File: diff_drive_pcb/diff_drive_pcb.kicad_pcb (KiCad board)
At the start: 2 copper layers, 13 parts, among them J1 Conn_01x02_Pin, J10 Conn_01x02_Pin, J2 Conn_01x04_Socket, J3 Conn_01x02_Pin, J4 Conn_01x04_Socket, J5 Conn_01x02_Pin, J6 Conn_01x04_Socket, J7 Conn_01x02_Pin, J8 Conn_01x04_Socket, J9 Conn_01x02_Pin, U1 TB6612FNG, U2 TB6612FNG, U3 Teensy4.1

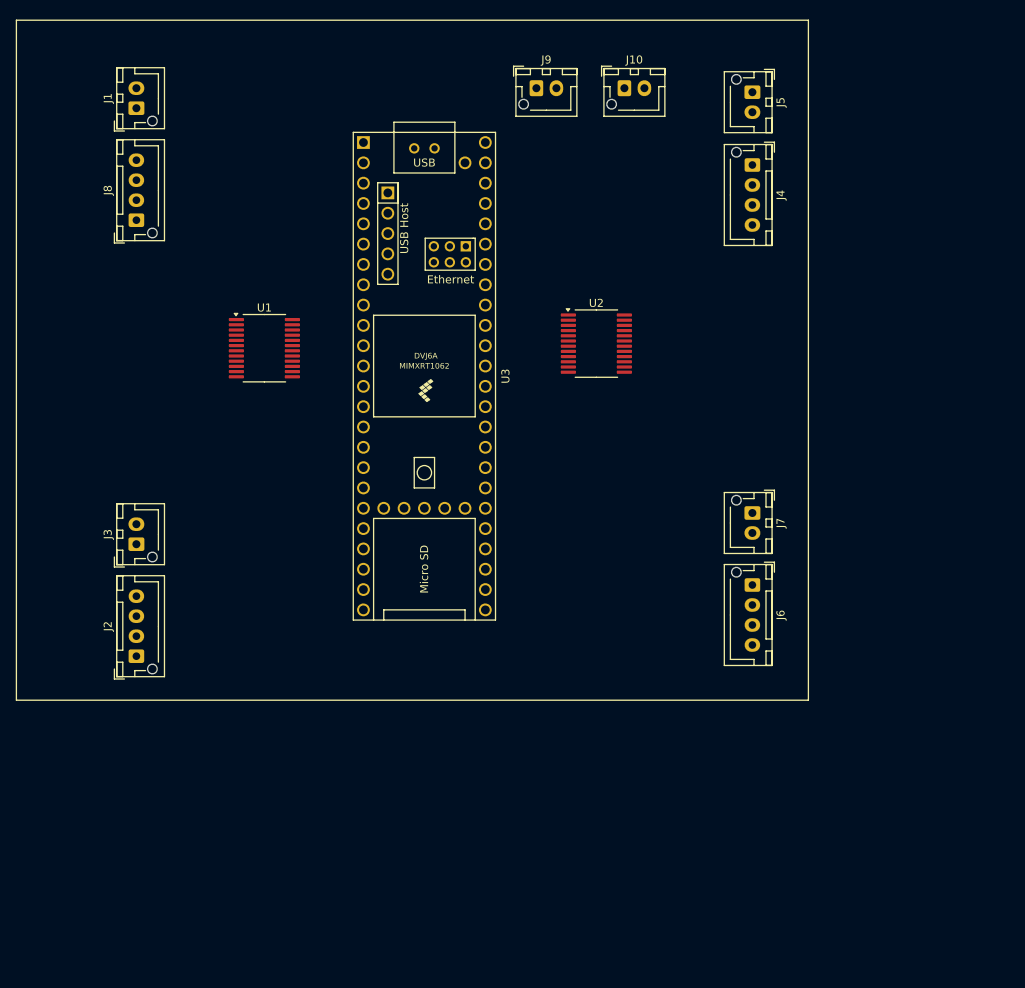
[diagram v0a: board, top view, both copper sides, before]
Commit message: PCB v1.0 developed
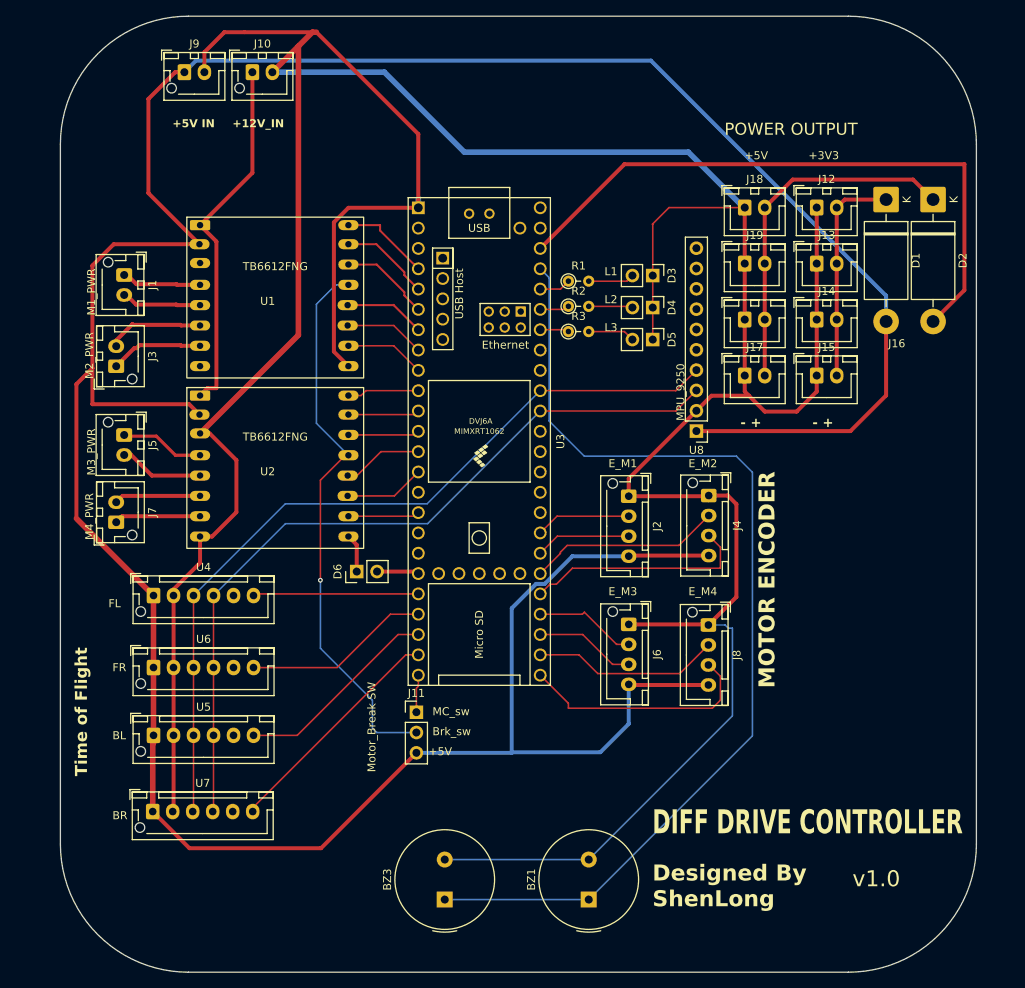
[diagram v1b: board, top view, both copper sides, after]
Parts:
- added BZ1: Buzzer, Buzzer_Beeper:Buzzer_TDK_PS1240P02BT_D12.2mm_H6.5mm, F.Cu at (167.5, 143.9)
- added BZ3: Buzzer, Buzzer_Beeper:Buzzer_TDK_PS1240P02BT_D12.2mm_H6.5mm, F.Cu at (149.5, 143.9)
- added D1: 1N5400, Diode_THT:D_DO-201AD_P15.24mm_Horizontal, F.Cu at (204.7, 56.4)
- added D2: 1N5400, Diode_THT:D_DO-201AD_P15.24mm_Horizontal, F.Cu at (210.6, 56.4)
- added D3: status_led1, Connector_PinHeader_2.54mm:PinHeader_1x02_P2.54mm_Vertical, F.Cu at (175.5, 65.9)
- added D4: status_led2, Connector_PinHeader_2.54mm:PinHeader_1x02_P2.54mm_Vertical, F.Cu at (175.5, 69.9)
- added D5: status_led3, Connector_PinHeader_2.54mm:PinHeader_1x02_P2.54mm_Vertical, F.Cu at (175.5, 73.9)
- added D6: headlight, Connector_PinHeader_2.54mm:PinHeader_1x02_P2.54mm_Vertical, F.Cu at (138.5, 102.9)
- added J11: Motor_Break_SW, Connector_PinHeader_2.54mm:PinHeader_1x03_P2.54mm_Vertical, F.Cu at (146.0, 120.5)
- added J12: 5v_out_1, Connector_JST:JST_XH_B2B-XH-A_1x02_P2.50mm_Vertical, F.Cu at (196.0, 57.4)
- added J13: 5v_out_2, Connector_JST:JST_XH_B2B-XH-A_1x02_P2.50mm_Vertical, F.Cu at (196.0, 64.4)
- added J14: 5v_out_3, Connector_JST:JST_XH_B2B-XH-A_1x02_P2.50mm_Vertical, F.Cu at (196.0, 71.4)
- added J15: 5v_out_4, Connector_JST:JST_XH_B2B-XH-A_1x02_P2.50mm_Vertical, F.Cu at (196.0, 78.4)
- added J16: 3v3_out_1, Connector_JST:JST_XH_B2B-XH-A_1x02_P2.50mm_Vertical, F.Cu at (187.0, 71.4)
- added J17: 3v3_out_2, Connector_JST:JST_XH_B2B-XH-A_1x02_P2.50mm_Vertical, F.Cu at (187.0, 78.4)
- added J18: 3v3_out_3, Connector_JST:JST_XH_B2B-XH-A_1x02_P2.50mm_Vertical, F.Cu at (187.0, 57.4)
- added J19: 3v3_out_4, Connector_JST:JST_XH_B2B-XH-A_1x02_P2.50mm_Vertical, F.Cu at (187.0, 64.4)
- added R1: 1K, Resistor_THT:R_Axial_DIN0204_L3.6mm_D1.6mm_P2.54mm_Vertical, F.Cu at (165.0, 66.6)
- added R2: 1K, Resistor_THT:R_Axial_DIN0204_L3.6mm_D1.6mm_P2.54mm_Vertical, F.Cu at (165.0, 69.8)
- added R3: 1K, Resistor_THT:R_Axial_DIN0204_L3.6mm_D1.6mm_P2.54mm_Vertical, F.Cu at (165.0, 72.9)
- added U4: TOF_front_left, Connector_JST:JST_XH_B6B-XH-AM_1x06_P2.50mm_Vertical, F.Cu at (113.1, 105.9)
- added U5: Tof_back_left, Connector_JST:JST_XH_B6B-XH-AM_1x06_P2.50mm_Vertical, F.Cu at (113.1, 123.4)
- added U6: Tof_front_right, Connector_JST:JST_XH_B6B-XH-AM_1x06_P2.50mm_Vertical, F.Cu at (113.1, 114.9)
- added U7: Tof_back_right, Connector_JST:JST_XH_B6B-XH-AM_1x06_P2.50mm_Vertical, F.Cu at (113.0, 132.9)
- added U8: MPU9250, Connector_PinHeader_2.54mm:PinHeader_1x10_P2.54mm_Vertical, F.Cu at (181.0, 85.4)
- J1: value Conn_01x02_Pin -> P_M1
- J10: value Conn_01x02_Pin -> 12V_IN
- J2: value Conn_01x04_Socket -> Encoder_M1
- J3: value Conn_01x02_Pin -> P_M2
- J4: value Conn_01x04_Socket -> Encoder_M2
- J5: value Conn_01x02_Pin -> P_M3
- J6: value Conn_01x04_Socket -> Encoder_M3
- J7: value Conn_01x02_Pin -> P_M4
- J8: value Conn_01x04_Socket -> Encoder_M4
- J9: value Conn_01x02_Pin -> 5V_IN
- U1: value TB6612FNG -> Motor Driver1; footprint Package_SO:SSOP-24_5.3x8.2mm_P0.65mm -> TB6612FNG:TB6612FNG breakout board
- U2: value TB6612FNG -> Motor Driver 2; footprint Package_SO:SSOP-24_5.3x8.2mm_P0.65mm -> TB6612FNG:TB6612FNG breakout board
- moved J5 89.5 mm to (109.5, 85.8)
- moved J8 87.6 mm to (182.5, 109.6), turned to -90 degrees
- moved J7 79.5 mm to (108.5, 96.8), turned to 90 degrees
- moved J2 64.7 mm to (172.5, 93.5), turned to -90 degrees
- moved J10 46.5 mm to (125.5, 40.5)
- moved J9 44.0 mm to (117.0, 40.5)
- moved U2 43.0 mm to (128.4, 90.0)
- moved J4 41.7 mm to (182.5, 93.4)
- moved J3 22.4 mm to (108.5, 77.2)
- moved J1 20.9 mm to (109.5, 65.8), turned to -90 degrees
- moved J6 16.2 mm to (172.5, 109.5)
- moved U3 10.7 mm to (153.9, 86.7)
- moved U1 6.47 mm to (128.4, 68.7)
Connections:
- U1 pad 1: /M1+ -> +12V
- U1 pad 10: Net-(U1-PGND2-Pad10) -> M1_ctrl_B
- U1 pad 11: /M2+ -> M1_ctrl_A
- U1 pad 12: /M2+ -> /Brk_sw
- U1 pad 13: unconnected-(U1-VM2-Pad13) -> M2_ctrl_A
- U1 pad 14: unconnected-(U1-VM3-Pad14) -> M2_ctrl_B
- U1 pad 15: unconnected-(U1-PWMB-Pad15) -> M2_ctrl_PWM
- U1 pad 16: unconnected-(U1-BIN2-Pad16) -> GND
- U1 pad 2: /M1+ -> +5V
- U1 pad 4: GND -> /M1+
- U1 pad 6: /M1- -> /M2-
- U1 pad 7: /M2- -> /M2+
- U1 pad 8: /M2- -> GND
- U1 pad 9: Net-(U1-PGND2-Pad10) -> M1_ctrl_PWM
- U2 pad 1: /M4+ -> +12V
- U2 pad 10: Net-(U2-PGND2-Pad10) -> M3_ctrl_B
- U2 pad 11: /M3+ -> M3_ctrl_A
- U2 pad 12: /M3+ -> /Brk_sw
- U2 pad 13: unconnected-(U2-VM2-Pad13) -> M4_ctrl_A
- U2 pad 14: unconnected-(U2-VM3-Pad14) -> M4_ctrl_B
- U2 pad 15: unconnected-(U2-PWMB-Pad15) -> M4_ctrl_PWM
- U2 pad 16: unconnected-(U2-BIN2-Pad16) -> GND
- U2 pad 2: /M4+ -> +5V
- U2 pad 4: GND -> /M3+
- U2 pad 5: /M4- -> /M3-
- U2 pad 7: /M3- -> /M4+
- U2 pad 8: /M3- -> GND
- U2 pad 9: Net-(U2-PGND2-Pad10) -> M3_ctrl_PWM
- U3 pad 10: M4_encB -> M3_ctrl_PWM
- U3 pad 11: M4_encA -> M3_ctrl_B
- U3 pad 12: unconnected-(U3-10_CS_MQSR-Pad12) -> M3_ctrl_A
- U3 pad 13: unconnected-(U3-11_MOSI_CTX1-Pad13) -> M4_ctrl_A
- U3 pad 14: unconnected-(U3-12_MISO_MQSL-Pad14) -> M4_ctrl_B
- U3 pad 16: unconnected-(U3-24_A10_TX6_SCL2-Pad16) -> M4_ctrl_PWM
- U3 pad 19: unconnected-(U3-27_A13_SCK1-Pad19) -> HEADLIGHTS
- U3 pad 20: unconnected-(U3-28_RX7-Pad20) -> XSHUT1
- U3 pad 21: unconnected-(U3-29_TX7-Pad21) -> XSHUT2
- U3 pad 22: unconnected-(U3-30_CRX3-Pad22) -> XSHUT3
- U3 pad 23: unconnected-(U3-31_CTX3-Pad23) -> XSHUT4
- U3 pad 24: unconnected-(U3-32_OUT1B-Pad24) -> /MD_stby
- U3 pad 25: unconnected-(U3-33_MCLK2-Pad25) -> M4_encA
- U3 pad 26: unconnected-(U3-34_RX8-Pad26) -> M4_encB
- U3 pad 27: unconnected-(U3-35_TX8-Pad27) -> M3_encA
- U3 pad 28: unconnected-(U3-36_CS-Pad28) -> M3_encB
- U3 pad 29: unconnected-(U3-37_CS-Pad29) -> M2_encA
- U3 pad 30: unconnected-(U3-38_CS1_IN1-Pad30) -> M2_encB
- U3 pad 31: unconnected-(U3-39_MISO1_OUT1A-Pad31) -> M1_encA
- U3 pad 32: unconnected-(U3-40_A16-Pad32) -> M1_encB
- U3 pad 38: unconnected-(U3-16_A2_RX4_SCL1-Pad38) -> MPU_SCL
- U3 pad 39: unconnected-(U3-17_A3_TX4_SDA1-Pad39) -> MPU_SDA
- U3 pad 4: M1_encB -> M1_ctrl_PWM
- U3 pad 42: unconnected-(U3-20_A6_TX5_LRCLK1-Pad42) -> STATUS_LED3
- U3 pad 43: unconnected-(U3-21_A7_RX5_BCLK1-Pad43) -> STATUS_LED2
- U3 pad 44: unconnected-(U3-22_A8_CTX1-Pad44) -> STATUS_LED1
- U3 pad 45: unconnected-(U3-23_A9_CRX1_MCLK1-Pad45) -> Buzzer_ctl
- U3 pad 46: unconnected-(U3-3V3-Pad46) -> +3V3
- U3 pad 5: M1_encA -> M1_ctrl_B
- U3 pad 6: M2_encB -> M1_ctrl_A
- U3 pad 7: M2_encA -> M2_ctrl_A
- U3 pad 8: M3_encB -> M2_ctrl_B
- U3 pad 9: M3_encA -> M2_ctrl_PWM
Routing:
- net GND: track 0.00 -> 466.7 mm
- net +5V: track 0.00 -> 399.4 mm
- net Buzzer_ctl: track 0.00 -> 127.4 mm
- net MPU_SDA: track 0.00 -> 101.6 mm
- net MPU_SCL: track 0.00 -> 98.0 mm
- net +3V3: track 0.00 -> 78.7 mm
- net /Brk_sw: track 0.00 -> 69.7 mm, vias 0 -> 1
- net +12V: track 0.00 -> 45.5 mm
- net Net-(D2-K): track 0.00 -> 44.5 mm
- net M4_encA: track 0.00 -> 30.2 mm
- net XSHUT4: track 0.00 -> 29.7 mm
- net M2_encA: track 0.00 -> 28.5 mm
- net Net-(D1-K): track 0.00 -> 27.6 mm
- net XSHUT3: track 0.00 -> 25.8 mm
- net M2_encB: track 0.00 -> 24.2 mm
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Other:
- board outline added: 114.5 x 119.5 mm
- board text added: "+12V_IN"
- board text added: "+3V3"
- board text added: "+5V"
- board text added: "+5V IN"
- board text added: "- +"
- board text added: "BL"
- board text added: "BR"
- board text added: "Brk_sw"
- board text added: "DIFF DRIVE CONTROLLER"
- board text added: "Designed By ShenLong"
- board text added: "E_M1"
- board text added: "E_M2"
- board text added: "E_M3"
- board text added: "E_M4"
- board text added: "FL"
- board text added: "FR"
- board text added: "L1"
- board text added: "L2"
- board text added: "L3"
- board text added: "M1_PWR"
- board text added: "M2_PWR"
- board text added: "M3_PWR"
- board text added: "M4_PWR"
- board text added: "MC_sw"
- board text added: "MOTOR ENCODER"
- board text added: "MPU_9250"
- board text added: "Motor_Break SW"
- board text added: "POWER OUTPUT"
- board text added: "Time of Flight"
- board text added: "v1.0"
